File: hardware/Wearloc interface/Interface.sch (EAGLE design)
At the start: 31 parts, among them J1 S4B-XH-A90°, J2 S4B-XH-A90°, J3 S3B-XH-A90°, J4 S6B-XH-A90°, U1 PCA9306DCT, U2 LTC2804-1GN, U3 TXB0104D, U4 MCP1826ADJ

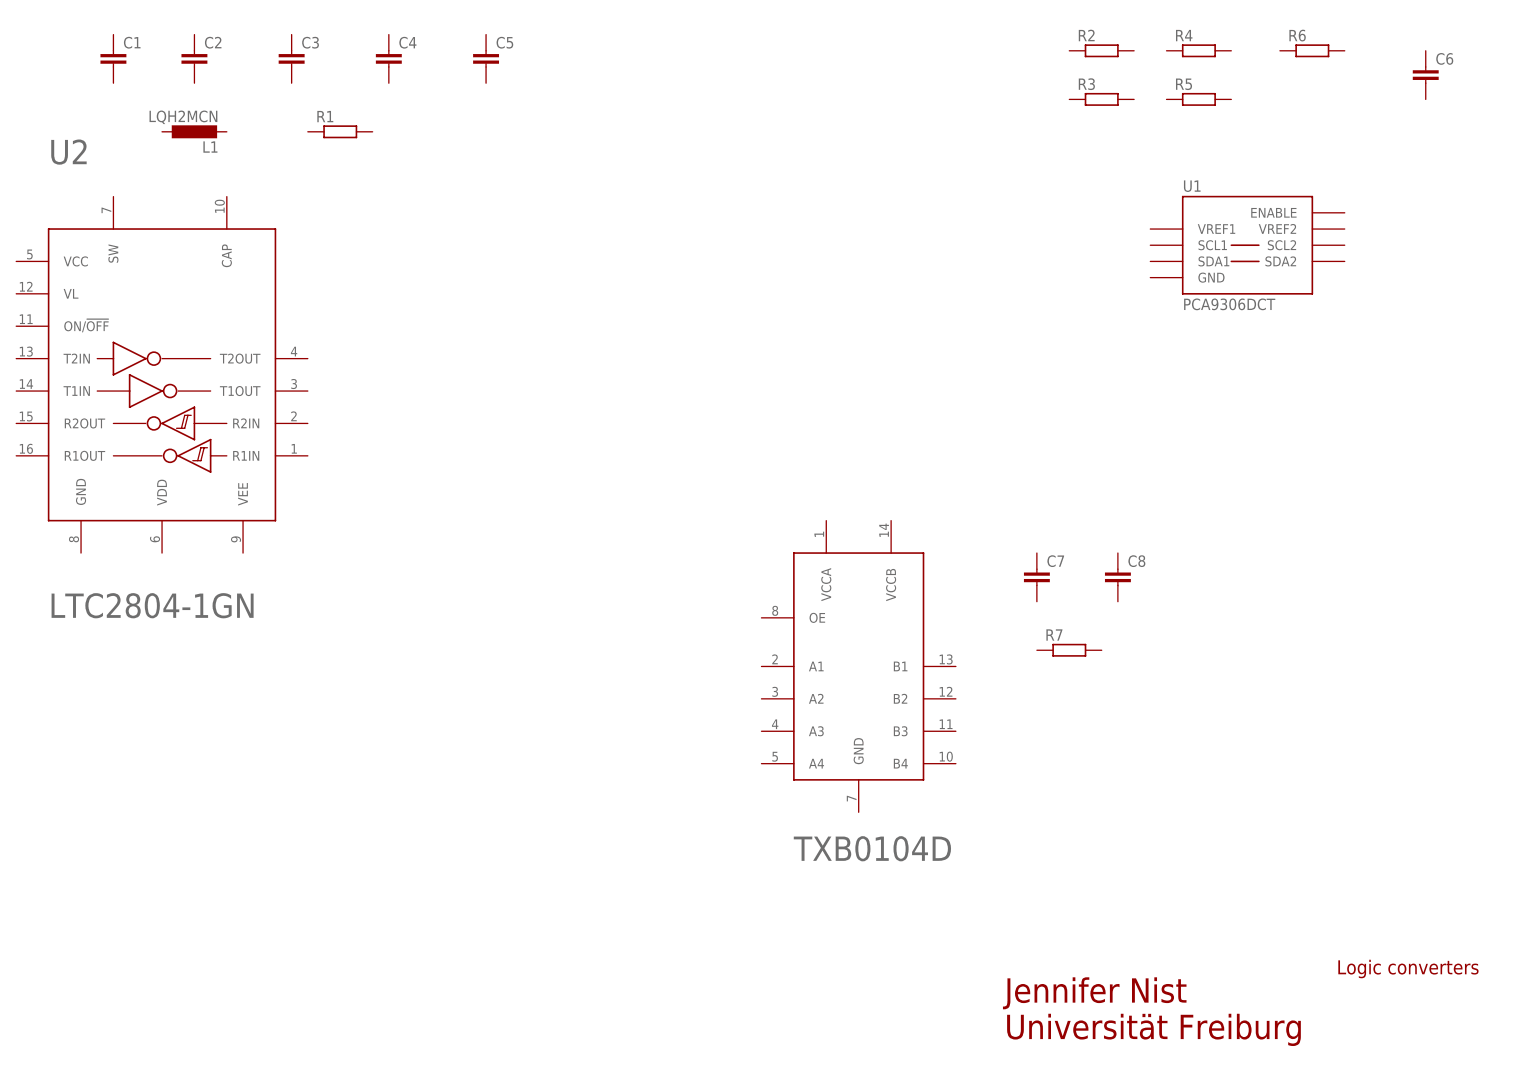
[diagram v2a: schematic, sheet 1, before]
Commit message: worked on schematic
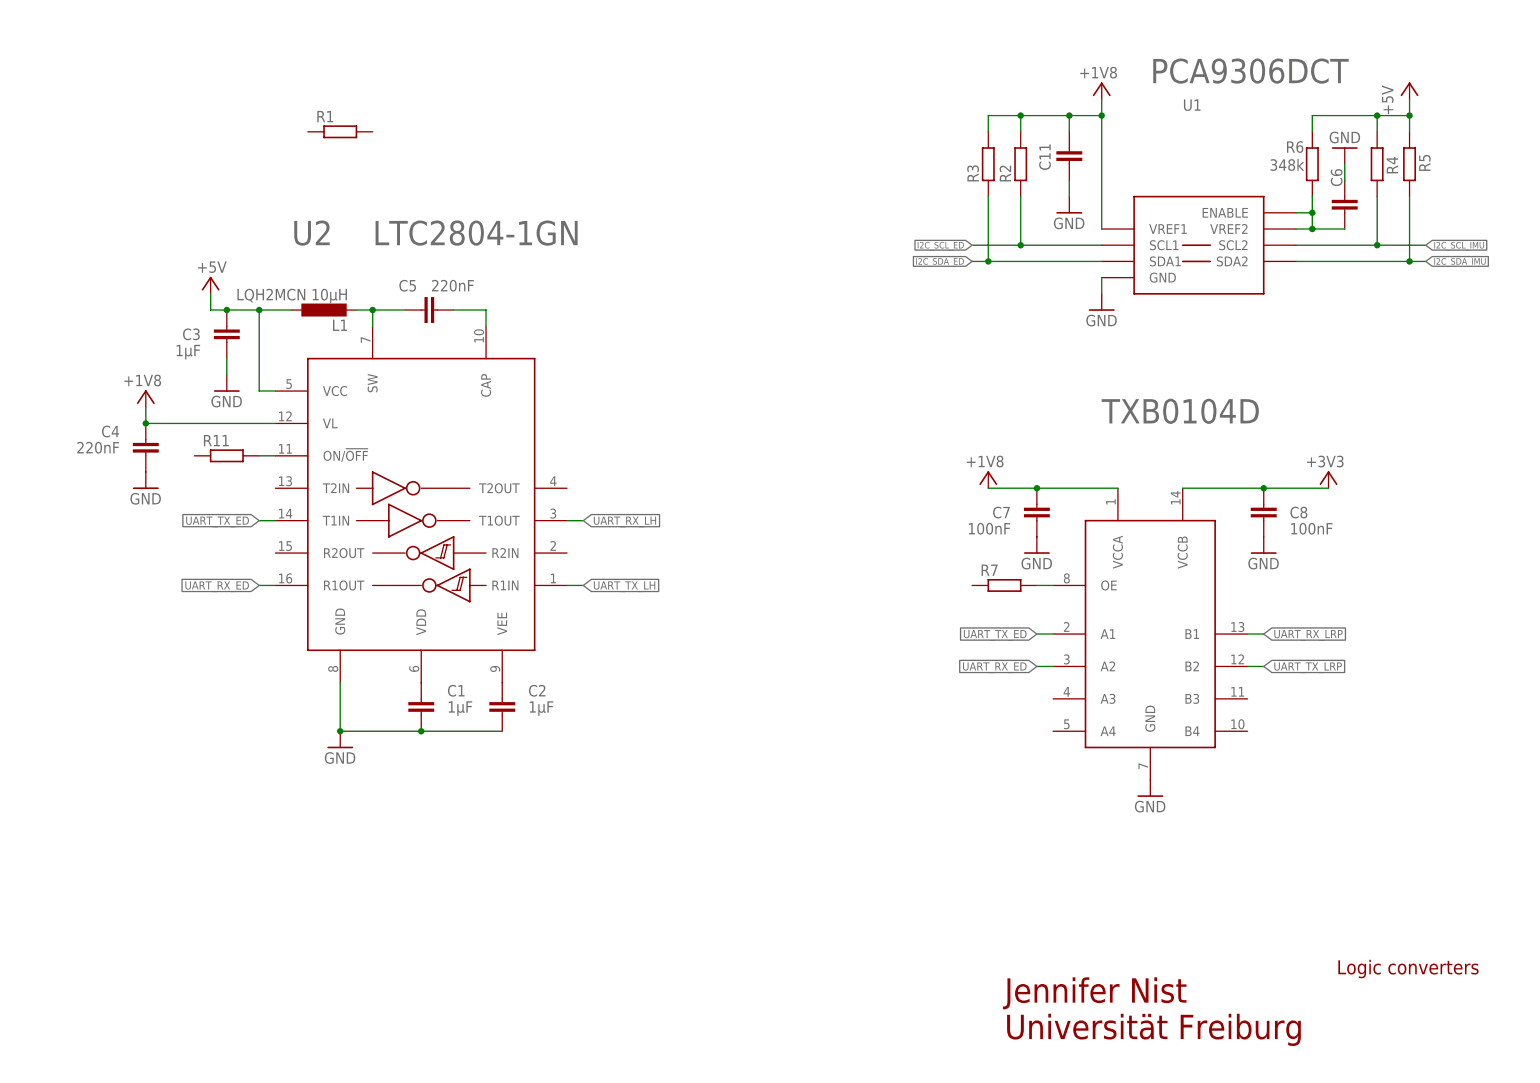
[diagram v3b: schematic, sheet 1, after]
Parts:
- removed J1: S4B-XH-A90°, wearloc:S4B-XH-A90°
- removed J4: S6B-XH-A90°, wearloc:S6B-XH-A90°
- added C11: (no value), rcl:C-EUC0805K
- added PH_IMU: S4B-XH-A90°, wearloc:S4B-XH-A90°
- added PH_LH: S6B-XH-A90°, wearloc:S6B-XH-A90°
- added R11: (no value), rcl:R-EU_R0805
- C1, C2, C3: value (none) -> 1µF
- C4, C5: value (none) -> 220nF
- C7, C8: value (none) -> 100nF
- L1: value LQH2MCN -> LQH2MCN 10µH
- R6: value (none) -> 348k
- renumbered J2 to PH2_LRP, J3 to PH1_LRP
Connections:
- new net I2C_SCL_ED: JP1J18.6, R2.2, U1.SCL1
- new net I2C_SCL_IMU: PH_IMU.1, R4.1, U1.SCL2
- new net I2C_SDA_ED: JP1J17.8, R3.2, U1.SDA1
- new net I2C_SDA_IMU: PH_IMU.2, R5.1, U1.SDA2
- new net N$3: R11.2, U2.ON/!OFF
- new net N$5: C5.1, L1.2, U2.SW
- new net N$6: C6.1, R6.1, U1.ENABLE, U1.VREF2
- new net N$7: C5.2, U2.CAP
- new net N$8: R7.2, U3.OE
- new net UART_RX_ED: JP1J18.13, U2.R1OUT, U3.A2
- new net UART_RX_LH: U2.T1OUT
- new net UART_RX_LRP: U3.B1
- new net UART_TX_ED: JP1J19.8, U2.T1IN, U3.A1
- new net UART_TX_LH: U2.R1IN
- new net UART_TX_LRP: U3.B2
- new net VDD: C1.1, U2.VDD
- new net VEE: C2.1, U2.VEE
- net +1V8: now also C11.2, C4.2, C7.1, R2.1, R3.1, U1.VREF1, U2.VL, U3.VCCA
- net +3V3: now also C8.1, U3.VCCB
- net +5V: now also C3.2, L1.1, PH_IMU.3, PH_LH.1, R4.2, R5.2, R6.2, U2.VCC
- net GND: now also C1.2, C11.1, C2.2, C3.1, C4.1, C6.2, C7.2, C8.2, JP1J19.3, PH_IMU.4, U1.GND, U2.GND, U3.GND
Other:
- moved on the sheet: C1, C2, C3, C4, C5, C6, C7, C8, JP1J17, JP1J18, JP1J19, JP1J20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
